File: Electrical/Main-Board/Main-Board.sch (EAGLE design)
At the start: 4 parts, among them IC1 ATMEGA16A-PU, J1 FTSH-105-01-L-DV-K-A-P-TR

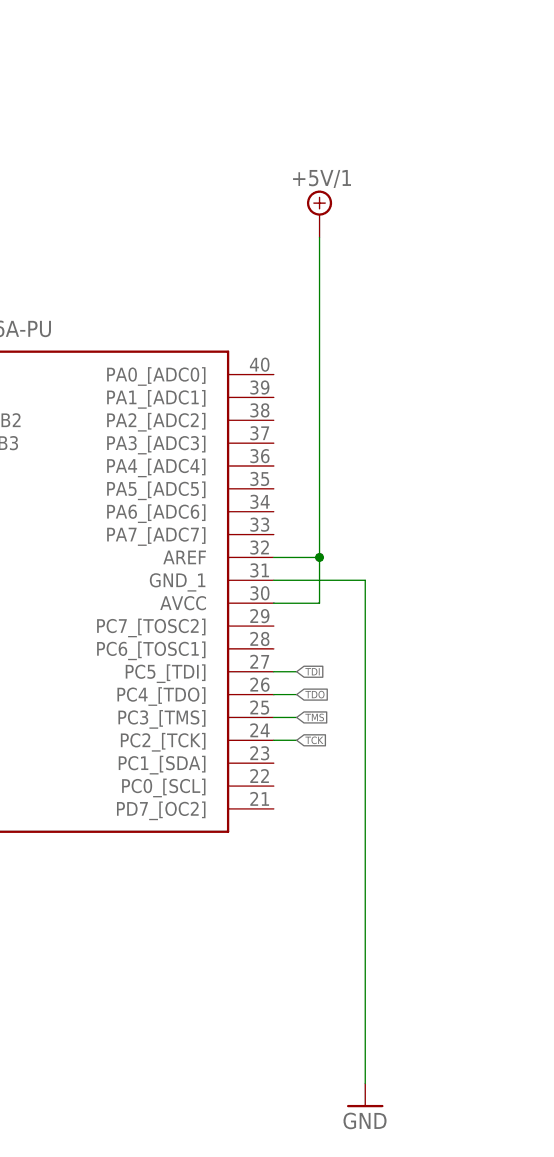
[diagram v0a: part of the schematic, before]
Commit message: Updated schematic
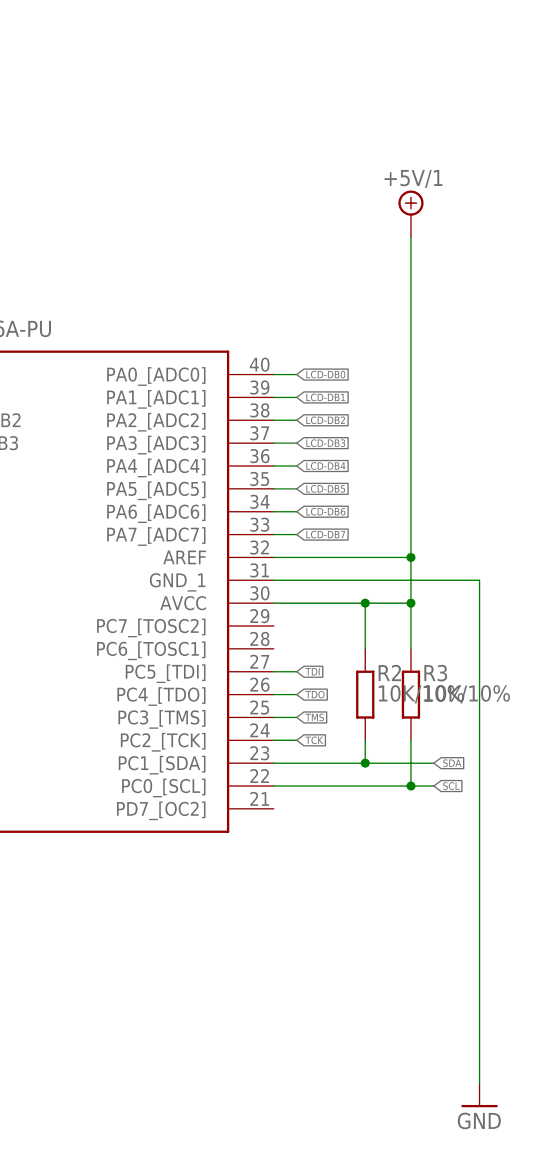
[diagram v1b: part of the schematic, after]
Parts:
- added R2, R3: 10K/10%, rcl:R-EU_R0603
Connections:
- new net LCD-DB0: IC1.PA0_[ADC0]
- new net LCD-DB1: IC1.PA1_[ADC1]
- new net LCD-DB2: IC1.PA2_[ADC2]
- new net LCD-DB3: IC1.PA3_[ADC3]
- new net LCD-DB4: IC1.PA4_[ADC4]
- new net LCD-DB5: IC1.PA5_[ADC5]
- new net LCD-DB6: IC1.PA6_[ADC6]
- new net LCD-DB7: IC1.PA7_[ADC7]
- new net SCL: IC1.PC0_[SCL], R3.1
- new net SDA: IC1.PC1_[SDA], R2.1
- net +5V/1: now also R2.2, R3.2
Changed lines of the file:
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@@
 <part name="S1" library="SamacSys_Parts" deviceset="PTS647SM50SMTR2LFS" device=""/>
 <part name="R1" library="rcl" library_urn="urn:adsk.eagle:library:334" deviceset="R-EU_" device="R0603" package3d_urn="urn:adsk.eagle:package:23555/3" value="10K/10%"/>
+<part name="R2" library="rcl" library_urn="urn:adsk.eagle:library:334" deviceset="R-EU_" device="R0603" package3d_urn="urn:adsk.eagle:package:23555/3" value="10K/10%"/>
+<part name="R3" library="rcl" library_urn="urn:adsk.eagle:library:334" deviceset="R-EU_" device="R0603" package3d_urn="urn:adsk.eagle:package:23555/3" value="10K/10%"/>
 </parts>
 <sheets>
@@
 <attribute name="VALUE" x="149.86" y="91.44" size="1.778" layer="96"/>
 </instance>
-<instance part="GND2" gate="1" x="220.98" y="93.98" smashed="yes">
-<attribute name="VALUE" x="218.44" y="91.44" size="1.778" layer="96"/>
-</instance>
-<instance part="SUPPLY1" gate="G$1" x="215.9" y="193.04" smashed="yes">
-<attribute name="VALUE" x="212.725" y="196.215" size="1.778" layer="96"/>
+<instance part="GND2" gate="1" x="233.68" y="93.98" smashed="yes">
+<attribute name="VALUE" x="231.14" y="91.44" size="1.778" layer="96"/>
+</instance>
+<instance part="SUPPLY1" gate="G$1" x="226.06" y="193.04" smashed="yes">
+<attribute name="VALUE" x="222.885" y="196.215" size="1.778" layer="96"/>
 </instance>
 <instance part="SUPPLY2" gate="G$1" x="152.4" y="193.04" smashed="yes">
@@
 <attribute name="NAME" x="140.97" y="164.0586" size="1.778" layer="95"/>
 <attribute name="VALUE" x="140.97" y="161.798" size="1.778" layer="96"/>
+</instance>
+<instance part="R2" gate="G$1" x="220.98" y="139.7" smashed="yes" rot="R90">
+<attribute name="NAME" x="222.25" y="141.1986" size="1.778" layer="95"/>
+<attribute name="VALUE" x="222.25" y="138.938" size="1.778" layer="96"/>
+</instance>
+<instance part="R3" gate="G$1" x="226.06" y="139.7" smashed="yes" rot="R90">
+<attribute name="NAME" x="227.33" y="141.1986" size="1.778" layer="95"/>
+<attribute name="VALUE" x="227.33" y="138.938" size="1.778" layer="96"/>
 </instance>
 </instances>
@@
 <pinref part="IC1" gate="G$1" pin="GND_1"/>
 <pinref part="GND2" gate="1" pin="GND"/>
-<wire x1="210.82" y1="152.4" x2="220.98" y2="152.4" width="0.1524" layer="91"/>
-<wire x1="220.98" y1="152.4" x2="220.98" y2="96.52" width="0.1524" layer="91"/>
+<wire x1="210.82" y1="152.4" x2="233.68" y2="152.4" width="0.1524" layer="91"/>
+<wire x1="233.68" y1="152.4" x2="233.68" y2="96.52" width="0.1524" layer="91"/>
 </segment>
 <segment>
@@
 <segment>
 <pinref part="IC1" gate="G$1" pin="AVCC"/>
-<wire x1="210.82" y1="149.86" x2="215.9" y2="149.86" width="0.1524" layer="91"/>
-<wire x1="215.9" y1="149.86" x2="215.9" y2="154.94" width="0.1524" layer="91"/>
+<wire x1="210.82" y1="149.86" x2="220.98" y2="149.86" width="0.1524" layer="91"/>
+<wire x1="220.98" y1="149.86" x2="226.06" y2="149.86" width="0.1524" layer="91"/>
+<wire x1="226.06" y1="149.86" x2="226.06" y2="154.94" width="0.1524" layer="91"/>
 <pinref part="IC1" gate="G$1" pin="AREF"/>
-<wire x1="215.9" y1="154.94" x2="210.82" y2="154.94" width="0.1524" layer="91"/>
-<wire x1="215.9" y1="154.94" x2="215.9" y2="190.5" width="0.1524" layer="91"/>
-<junction x="215.9" y="154.94"/>
+<wire x1="226.06" y1="154.94" x2="210.82" y2="154.94" width="0.1524" layer="91"/>
+<wire x1="226.06" y1="154.94" x2="226.06" y2="190.5" width="0.1524" layer="91"/>
+<junction x="226.06" y="154.94"/>
 <pinref part="SUPPLY1" gate="G$1" pin="+5V/1"/>
+<pinref part="R2" gate="G$1" pin="2"/>
+<wire x1="220.98" y1="144.78" x2="220.98" y2="149.86" width="0.1524" layer="91"/>
+<junction x="220.98" y="149.86"/>
+<pinref part="R3" gate="G$1" pin="2"/>
+<wire x1="226.06" y1="144.78" x2="226.06" y2="149.86" width="0.1524" layer="91"/>
+<junction x="226.06" y="149.86"/>
 </segment>
 <segment>
@@
 </segment>
 </net>
+<net name="SDA" class="0">
+<segment>
+<pinref part="IC1" gate="G$1" pin="PC1_[SDA]"/>
+<wire x1="210.82" y1="132.08" x2="220.98" y2="132.08" width="0.1524" layer="91"/>
+<label x="228.6" y="132.08" size="0.8128" layer="95" xref="yes"/>
+<pinref part="R2" gate="G$1" pin="1"/>
+<wire x1="220.98" y1="132.08" x2="228.6" y2="132.08" width="0.1524" layer="91"/>
+<wire x1="220.98" y1="134.62" x2="220.98" y2="132.08" width="0.1524" layer="91"/>
+<junction x="220.98" y="132.08"/>
+</segment>
+</net>
+<net name="SCL" class="0">
+<segment>
+<pinref part="IC1" gate="G$1" pin="PC0_[SCL]"/>
+<wire x1="210.82" y1="129.54" x2="226.06" y2="129.54" width="0.1524" layer="91"/>
+<label x="228.6" y="129.54" size="0.8128" layer="95" xref="yes"/>
+<pinref part="R3" gate="G$1" pin="1"/>
+<wire x1="226.06" y1="129.54" x2="228.6" y2="129.54" width="0.1524" layer="91"/>
+<wire x1="226.06" y1="134.62" x2="226.06" y2="129.54" width="0.1524" layer="91"/>
+<junction x="226.06" y="129.54"/>
+</segment>
+</net>
+<net name="LCD-DB0" class="0">
+<segment>
+<pinref part="IC1" gate="G$1" pin="PA0_[ADC0]"/>
+<wire x1="210.82" y1="175.26" x2="213.36" y2="175.26" width="0.1524" layer="91"/>
+<label x="213.36" y="175.26" size="0.8128" layer="95" xref="yes"/>
+</segment>
+</net>
+<net name="LCD-DB1" class="0">
+<segment>
+<pinref part="IC1" gate="G$1" pin="PA1_[ADC1]"/>
+<wire x1="210.82" y1="172.72" x2="213.36" y2="172.72" width="0.1524" layer="91"/>
+<label x="213.36" y="172.72" size="0.8128" layer="95" xref="yes"/>
+</segment>
+</net>
+<net name="LCD-DB2" class="0">
+<segment>
+<pinref part="IC1" gate="G$1" pin="PA2_[ADC2]"/>
+<wire x1="210.82" y1="170.18" x2="213.36" y2="170.18" width="0.1524" layer="91"/>
+<label x="213.36" y="170.18" size="0.8128" layer="95" xref="yes"/>
+</segment>
+</net>
+<net name="LCD-DB3" class="0">
+<segment>
+<pinref part="IC1" gate="G$1" pin="PA3_[ADC3]"/>
+<wire x1="210.82" y1="167.64" x2="213.36" y2="167.64" width="0.1524" layer="91"/>
+<label x="213.36" y="167.64" size="0.8128" layer="95" xref="yes"/>
+</segment>
+</net>
+<net name="LCD-DB4" class="0">
+<segment>
+<pinref part="IC1" gate="G$1" pin="PA4_[ADC4]"/>
+<wire x1="210.82" y1="165.1" x2="213.36" y2="165.1" width="0.1524" layer="91"/>
+<label x="213.36" y="165.1" size="0.8128" layer="95" xref="yes"/>
+</segment>
+</net>
+<net name="LCD-DB5" class="0">
+<segment>
+<pinref part="IC1" gate="G$1" pin="PA5_[ADC5]"/>
+<wire x1="210.82" y1="162.56" x2="213.36" y2="162.56" width="0.1524" layer="91"/>
+<label x="213.36" y="162.56" size="0.8128" layer="95" xref="yes"/>
+</segment>
+</net>
+<net name="LCD-DB6" class="0">
+<segment>
+<pinref part="IC1" gate="G$1" pin="PA6_[ADC6]"/>
+<wire x1="210.82" y1="160.02" x2="213.36" y2="160.02" width="0.1524" layer="91"/>
+<label x="213.36" y="160.02" size="0.8128" layer="95" xref="yes"/>
+</segment>
+</net>
+<net name="LCD-DB7" class="0">
+<segment>
+<pinref part="IC1" gate="G$1" pin="PA7_[ADC7]"/>
+<wire x1="210.82" y1="157.48" x2="213.36" y2="157.48" width="0.1524" layer="91"/>
+<label x="213.36" y="157.48" size="0.8128" layer="95" xref="yes"/>
+</segment>
+</net>
